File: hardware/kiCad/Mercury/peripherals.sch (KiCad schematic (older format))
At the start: 48 parts, among them J13 5-1814832-1, J14 5-1814832-1, U4 MPU-6050, U5 W25N01GVZEIG_TR, U6 LPS25HB, U7 CC2500, U8 CC2592RGVR, U9 MAX-8Q, Y2 26 MHz Oscillator

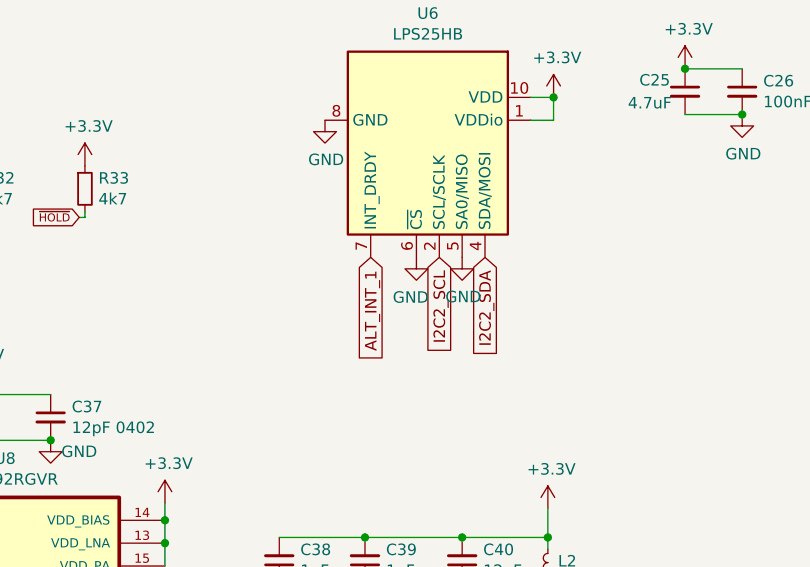
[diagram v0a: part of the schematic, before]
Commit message: Updated with final board design
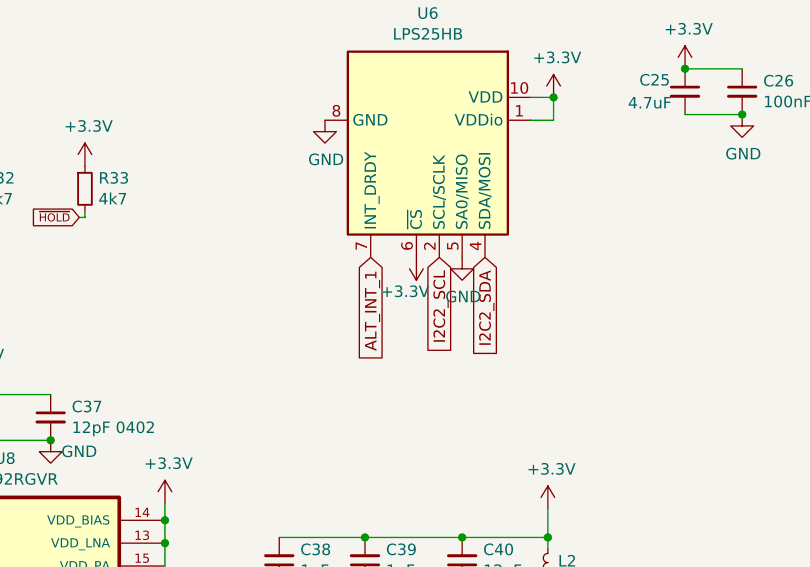
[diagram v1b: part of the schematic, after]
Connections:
- net +3V3: now also U6.6 (~CS)
- net GND: no longer U6.6 (~CS)
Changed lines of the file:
@@
 	1    0    0    -1
 $EndComp
-Text GLabel 3750 1400 0    50   Input ~ 0
-FLASH_CS
 $Comp
 L power:+3.3V #PWR0161
@@
 	1    0    0    -1
 $EndComp
-Text GLabel 3750 1700 0    50   Input ~ 0
-SPI2_MOSI
-Text GLabel 3750 1800 0    50   Input ~ 0
-SPI2_MISO
-Text GLabel 3750 1500 0    50   Input ~ 0
-SPI2_SCK
 $Comp
 L RF_GPS:MAX-8Q U9
@@
 Wire Wire Line
 	1325 7150 1350 7150
+Wire Wire Line
+	8900 1175 8900 1275
+Connection ~ 8900 1175
+$Comp
+L power:GND #PWR0128
+U 1 1 5FFAFB5B
+P 8500 1875
+F 0 "#PWR0128" H 8500 1625 50  0001 C CNN
+F 1 "GND" H 8505 1702 50  0000 C CNN
+F 2 "" H 8500 1875 50  0001 C CNN
+F 3 "" H 8500 1875 50  0001 C CNN
+	1    8500 1875
+	1    0    0    -1
+$EndComp
+Connection ~ 9725 1250
+Wire Wire Line
+	9475 1250 9725 1250
+Wire Wire Line
+	9475 1050 9725 1050
+$Comp
+L Device:C_Small C25
+U 1 1 5FEC8637
+P 9475 1150
+F 0 "C25" H 9275 1200 50  0000 L CNN
+F 1 "4.7uF" H 9225 1100 50  0000 L CNN
+F 2 "Capacitor_SMD:C_0805_2012Metric" H 9475 1150 50  0001 C CNN
+F 3 "~" H 9475 1150 50  0001 C CNN
+	1    9475 1150
+	1    0    0    -1
+$EndComp
+$Comp
+L power:GND #PWR0155
+U 1 1 5FEC6232
+P 9725 1250
+F 0 "#PWR0155" H 9725 1000 50  0001 C CNN
+F 1 "GND" H 9730 1077 50  0000 C CNN
+F 2 "" H 9725 1250 50  0001 C CNN
+F 3 "" H 9725 1250 50  0001 C CNN
+	1    9725 1250
+	1    0    0    -1
+$EndComp
+$Comp
+L Device:C_Small C26
+U 1 1 5FEC6044
+P 9725 1150
+F 0 "C26" H 9817 1196 50  0000 L CNN
+F 1 "100nF" H 9817 1105 50  0000 L CNN
+F 2 "Capacitor_SMD:C_0603_1608Metric" H 9725 1150 50  0001 C CNN
+F 3 "~" H 9725 1150 50  0001 C CNN
+	1    9725 1150
+	1    0    0    -1
+$EndComp
+$Comp
+L Sensor_Pressure:LPS25HB U6
+U 1 1 6002FC1C
+P 8400 1375
+F 0 "U6" V 7833 1325 50  0000 C CNN
+F 1 "LPS25HB" V 7924 1325 50  0000 C CNN
+F 2 "Package_LGA:ST_HLGA-10_2.5x2.5mm_P0.6mm_LayoutBorder3x2y" H 8400 1175 50  0001 C CNN
+F 3 "www.st.com/resource/en/datasheet/lps25hb.pdf" H 8450 1025 50  0001 C CNN
+	1    8400 1375
+	0    1    1    0
+$EndComp
+Wire Wire Line
+	8800 1175 8900 1175
+Wire Wire Line
+	8800 1275 8900 1275
+$Comp
+L power:+3.3V #PWR0130
+U 1 1 6006B3D3
+P 9475 1050
+F 0 "#PWR0130" H 9475 900 50  0001 C CNN
+F 1 "+3.3V" H 9490 1223 50  0000 C CNN
+F 2 "" H 9475 1050 50  0001 C CNN
+F 3 "" H 9475 1050 50  0001 C CNN
+	1    9475 1050
+	1    0    0    -1
+$EndComp
+Connection ~ 9475 1050
+Wire Wire Line
+	1200 2800 1200 2825
+Wire Wire Line
+	1200 2800 1600 2800
+Connection ~ 1200 2800
+Connection ~ 1600 2800
+$Comp
+L power:GND #PWR0131
+U 1 1 5FF89171
+P 6700 2675
+F 0 "#PWR0131" H 6700 2425 50  0001 C CNN
+F 1 "GND" H 6825 2625 50  0000 C CNN
+F 2 "" H 6700 2675 50  0001 C CNN
+F 3 "" H 6700 2675 50  0001 C CNN
+	1    6700 2675
+	1    0    0    -1
+$EndComp
+Connection ~ 6700 2675
+$Comp
+L power:+3.3V #PWR0129
+U 1 1 5FF9862B
+P 8300 1875
+F 0 "#PWR0129" H 8300 1725 50  0001 C CNN
+F 1 "+3.3V" H 8350 2025 50  0000 C CNN
+F 2 "" H 8300 1875 50  0001 C CNN
+F 3 "" H 8300 1875 50  0001 C CNN
+	1    8300 1875
+	-1   0    0    1
+$EndComp
 $Comp
 L W25N01GVZEIG:W25N01GVZEIG_TR U5
@@
 	1    0    0    -1
 $EndComp
-Wire Wire Line
-	8900 1175 8900 1275
-Connection ~ 8900 1175
-$Comp
-L power:GND #PWR0128
-U 1 1 5FFAFB5B
-P 8500 1875
-F 0 "#PWR0128" H 8500 1625 50  0001 C CNN
-F 1 "GND" H 8505 1702 50  0000 C CNN
-F 2 "" H 8500 1875 50  0001 C CNN
-F 3 "" H 8500 1875 50  0001 C CNN
-	1    8500 1875
-	1    0    0    -1
-$EndComp
-Connection ~ 9725 1250
-Wire Wire Line
-	9475 1250 9725 1250
-Wire Wire Line
-	9475 1050 9725 1050
-$Comp
-L Device:C_Small C25
-U 1 1 5FEC8637
-P 9475 1150
-F 0 "C25" H 9275 1200 50  0000 L CNN
-F 1 "4.7uF" H 9225 1100 50  0000 L CNN
-F 2 "Capacitor_SMD:C_0805_2012Metric" H 9475 1150 50  0001 C CNN
-F 3 "~" H 9475 1150 50  0001 C CNN
-	1    9475 1150
-	1    0    0    -1
-$EndComp
-$Comp
-L power:GND #PWR0155
-U 1 1 5FEC6232
-P 9725 1250
-F 0 "#PWR0155" H 9725 1000 50  0001 C CNN
-F 1 "GND" H 9730 1077 50  0000 C CNN
-F 2 "" H 9725 1250 50  0001 C CNN
-F 3 "" H 9725 1250 50  0001 C CNN
-	1    9725 1250
-	1    0    0    -1
-$EndComp
-$Comp
-L Device:C_Small C26
-U 1 1 5FEC6044
-P 9725 1150
-F 0 "C26" H 9817 1196 50  0000 L CNN
-F 1 "100nF" H 9817 1105 50  0000 L CNN
-F 2 "Capacitor_SMD:C_0603_1608Metric" H 9725 1150 50  0001 C CNN
-F 3 "~" H 9725 1150 50  0001 C CNN
-	1    9725 1150
-	1    0    0    -1
-$EndComp
-$Comp
-L Sensor_Pressure:LPS25HB U6
-U 1 1 6002FC1C
-P 8400 1375
-F 0 "U6" V 7833 1325 50  0000 C CNN
-F 1 "LPS25HB" V 7924 1325 50  0000 C CNN
-F 2 "Package_LGA:ST_HLGA-10_2.5x2.5mm_P0.6mm_LayoutBorder3x2y" H 8400 1175 50  0001 C CNN
-F 3 "www.st.com/resource/en/datasheet/lps25hb.pdf" H 8450 1025 50  0001 C CNN
-	1    8400 1375
-	0    1    1    0
-$EndComp
-Wire Wire Line
-	8800 1175 8900 1175
-Wire Wire Line
-	8800 1275 8900 1275
-$Comp
-L power:GND #PWR0129
-U 1 1 600485C8
-P 8300 1875
-F 0 "#PWR0129" H 8300 1625 50  0001 C CNN
-F 1 "GND" H 8275 1700 50  0000 C CNN
-F 2 "" H 8300 1875 50  0001 C CNN
-F 3 "" H 8300 1875 50  0001 C CNN
-	1    8300 1875
-	1    0    0    -1
-$EndComp
-$Comp
-L power:+3.3V #PWR0130
-U 1 1 6006B3D3
-P 9475 1050
-F 0 "#PWR0130" H 9475 900 50  0001 C CNN
-F 1 "+3.3V" H 9490 1223 50  0000 C CNN
-F 2 "" H 9475 1050 50  0001 C CNN
-F 3 "" H 9475 1050 50  0001 C CNN
-	1    9475 1050
-	1    0    0    -1
-$EndComp
-Connection ~ 9475 1050
-Wire Wire Line
-	1200 2800 1200 2825
-Wire Wire Line
-	1200 2800 1600 2800
-Connection ~ 1200 2800
-Connection ~ 1600 2800
-$Comp
-L power:GND #PWR?
-U 1 1 5FF89171
-P 6700 2675
-F 0 "#PWR?" H 6700 2425 50  0001 C CNN
-F 1 "GND" H 6825 2625 50  0000 C CNN
-F 2 "" H 6700 2675 50  0001 C CNN
-F 3 "" H 6700 2675 50  0001 C CNN
-	1    6700 2675
-	1    0    0    -1
-$EndComp
-Connection ~ 6700 2675
+Text GLabel 3750 1500 0    50   Input ~ 0
+SPI2_SCK
+Text GLabel 3750 1800 0    50   Input ~ 0
+SPI2_MISO
+Text GLabel 3750 1700 0    50   Input ~ 0
+SPI2_MOSI
+Text GLabel 3750 1400 0    50   Input ~ 0
+FLASH_CS
 $EndSCHEMATC
